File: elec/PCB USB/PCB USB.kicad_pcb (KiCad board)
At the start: 2 copper layers, 91 x 38 mm, 99 parts, among them J201 USB_C_PICO, J402 USB_C_Receptacle_USB2.0_14P, J403 USB_A, J404 USB_C_Receptacle_USB2.0_14P, J405 USB_A, J501 Conn_I2C_Écran, P1 USB_C_Plug_USB2.0, Q301 AO3401A, Q401 AO3401A, SW201 SW_BOOTSEL, SW202 SW_RESET, SW501 RotaryEncoder_Switch, U201 SRV05-4, U202 RP2350B-QFN80, U203 W25Q128JVPIQ, U301 AP7361C-33E, U401 SRV05-4, Y201 CM4012M00012001, Y401 12MHz

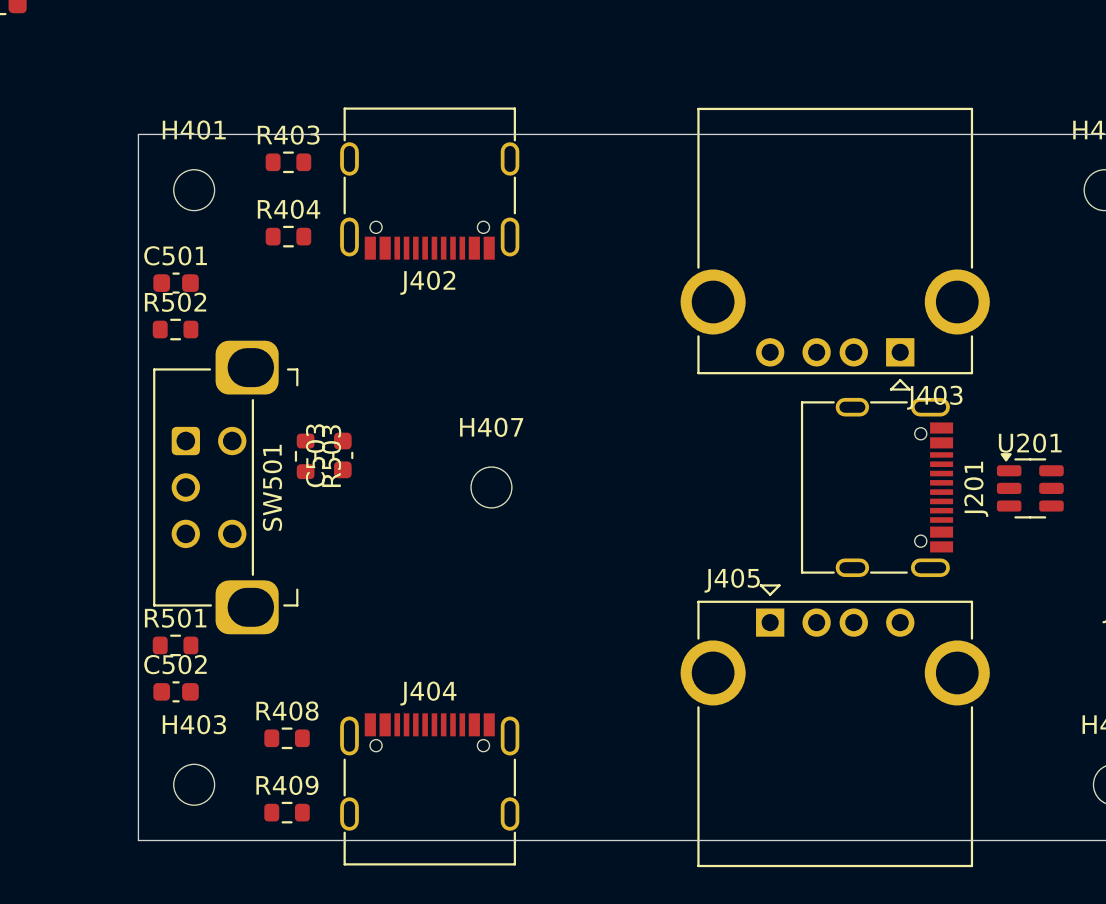
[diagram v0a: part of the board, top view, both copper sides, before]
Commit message: speed
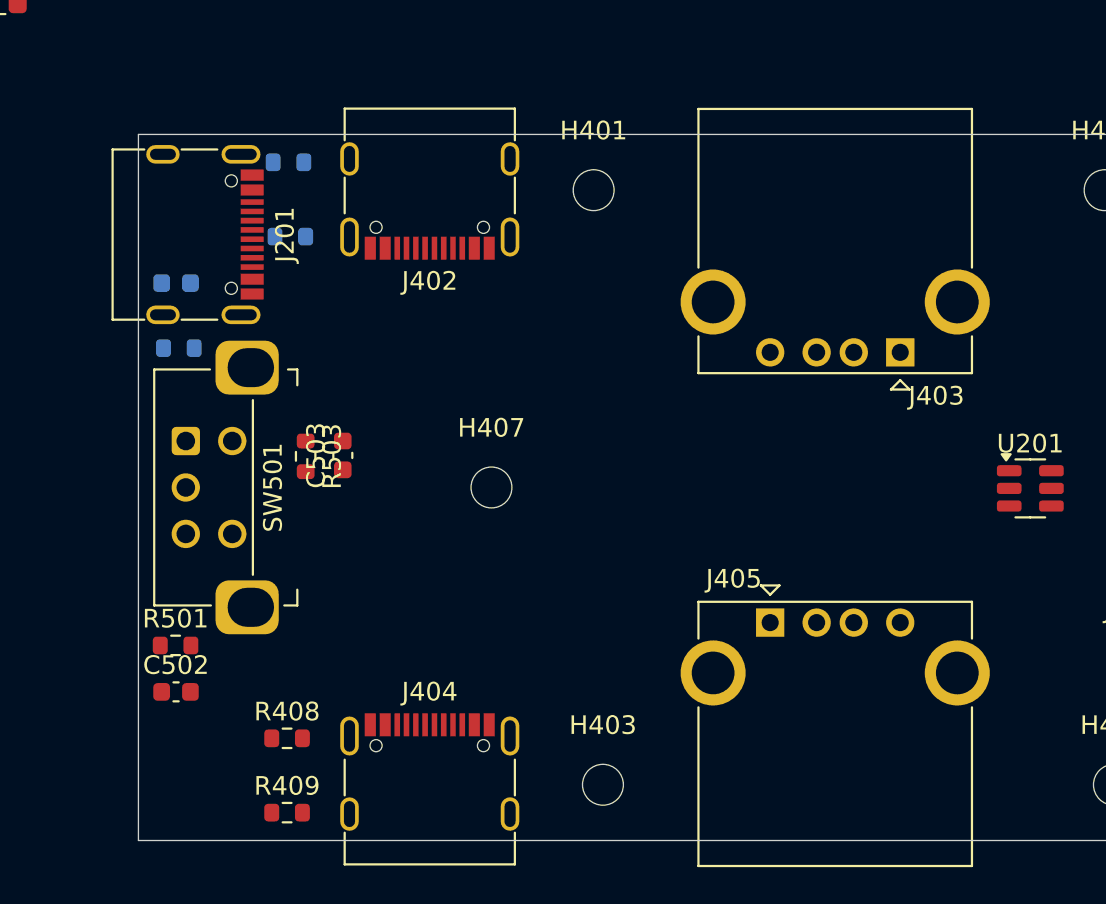
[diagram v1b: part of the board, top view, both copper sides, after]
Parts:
- C501, R403, R404, R502: moved to B.Cu
- moved J201 39.5 mm to (86.9, 84.4)
- moved H403 22.0 mm to (109.5, 114.0)
- moved H401 21.5 mm to (109.0, 82.0)
- moved R502 1.02 mm to (86.7, 90.5), turned to 180 degrees
- moved R404 0.10 mm to (92.7, 84.5), turned to 180 degrees
- turned C501 to 180 degrees
- turned R403 to 180 degrees
